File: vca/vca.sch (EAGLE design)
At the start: 59 parts, among them IC1 OPA4130U, IC2 OPA134D, Q1 BC847ALT1SMD, X1 2516-

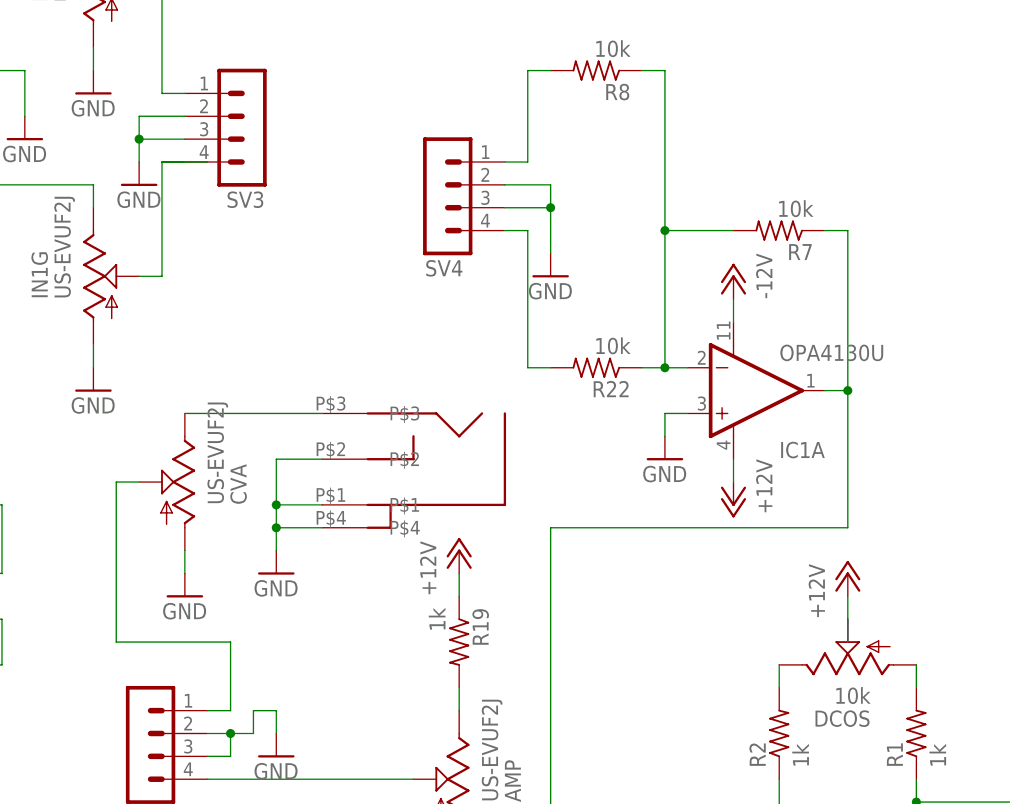
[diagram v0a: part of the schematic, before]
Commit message: sent out vca again
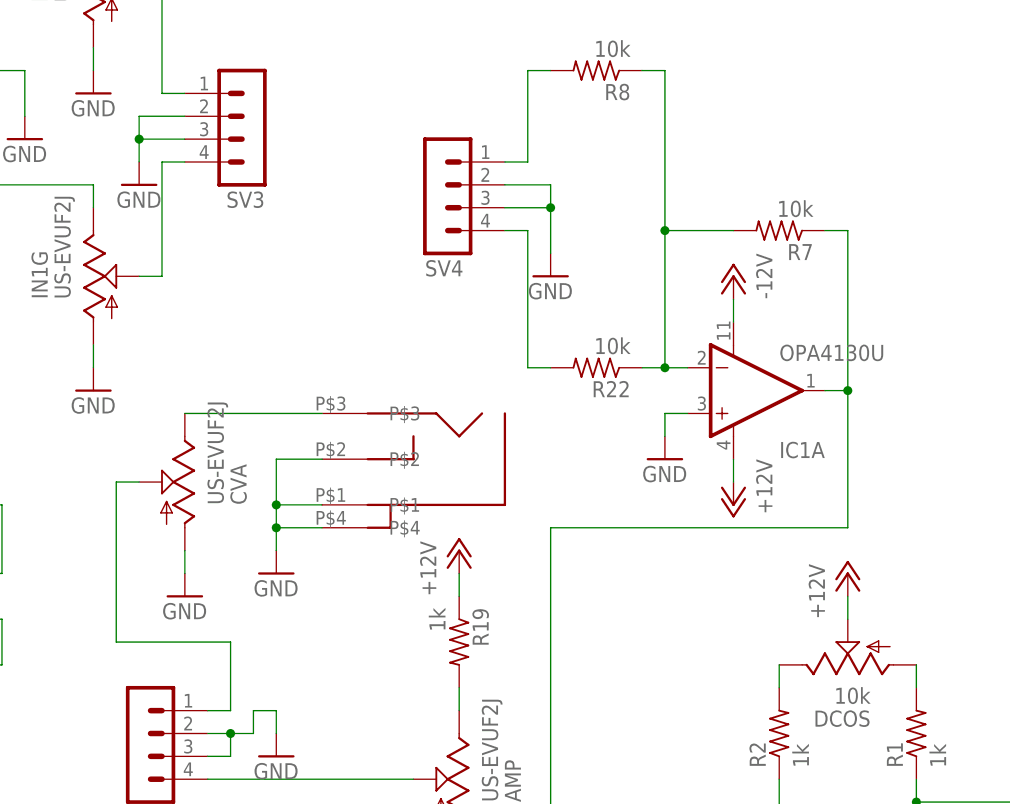
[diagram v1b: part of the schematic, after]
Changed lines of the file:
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@@
-</segment>
-<segment>
-<wire x1="-40.64" y1="129.54" x2="-45.72" y2="129.54" width="0.1524" layer="91"/>
 </segment>
 <segment>
@@
 <pinref part="P+3" gate="1" pin="+12V"/>
 <wire x1="30.48" y1="78.74" x2="30.48" y2="81.28" width="0.1524" layer="91"/>
-<wire x1="30.48" y1="76.2" x2="30.48" y2="78.74" width="0.1524" layer="91"/>
 </segment>
 <segment>
